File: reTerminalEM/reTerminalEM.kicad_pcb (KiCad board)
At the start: 2 copper layers, 135 x 90 mm, 7 parts, among them J1 FX23-100S-0.5SV

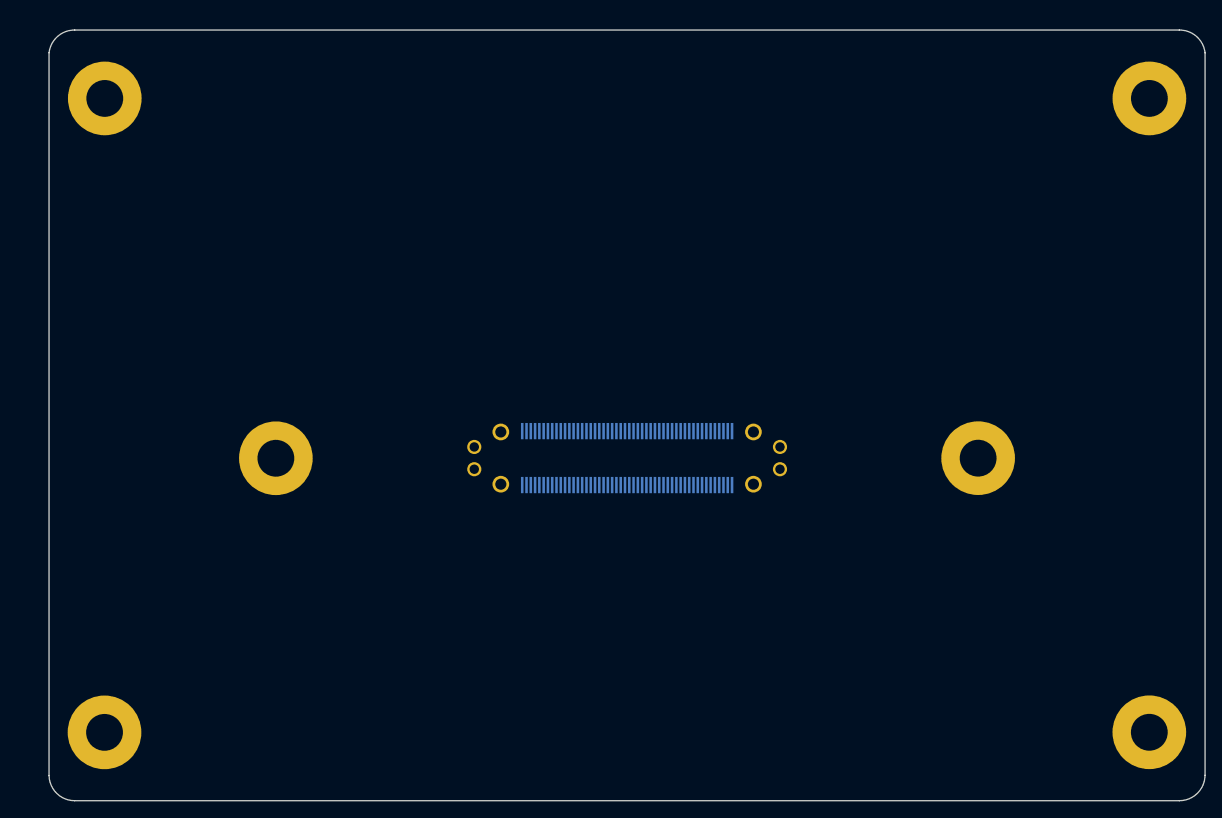
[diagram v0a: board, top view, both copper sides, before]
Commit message: fixing dimensions, adding .step, .dxf, .pdf
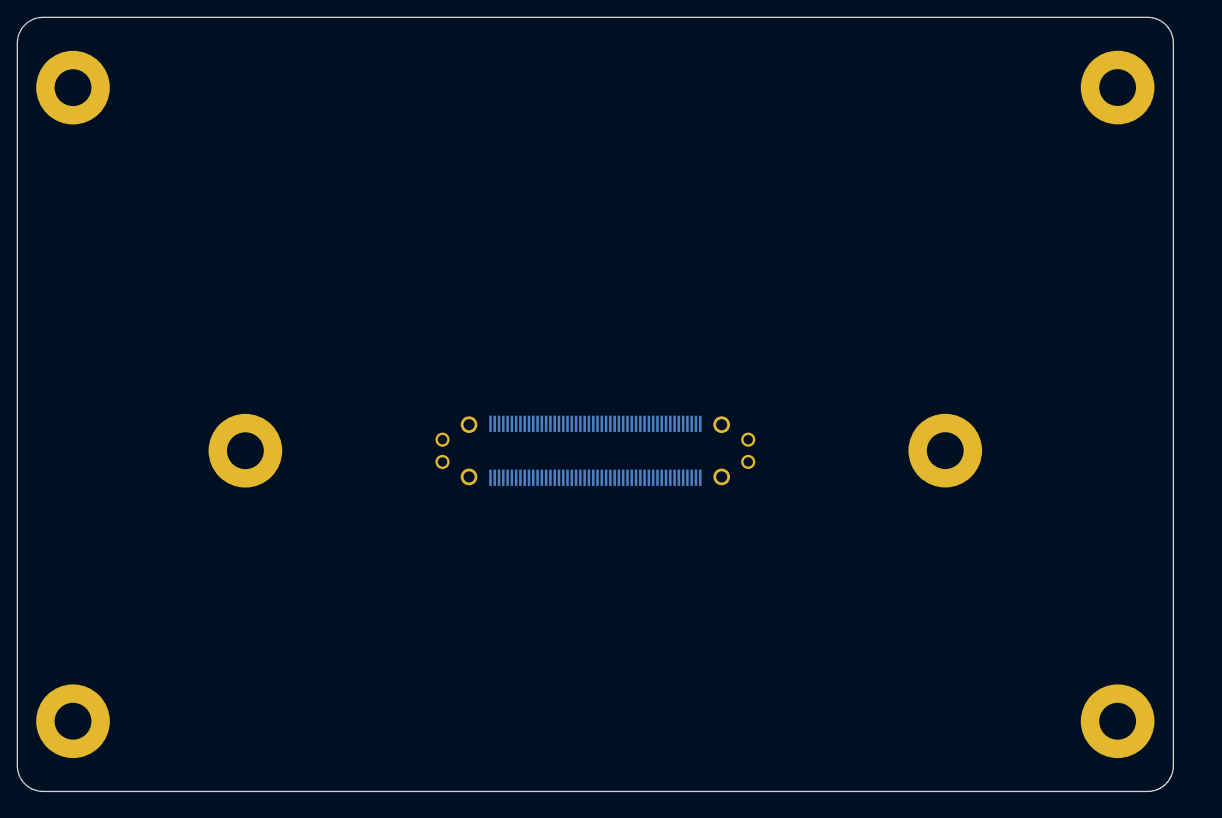
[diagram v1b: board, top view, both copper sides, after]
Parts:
- removed the REF** at (214.3, 136.8)
- removed the REF** at (214.3, 62.8)
- added REF**: MountingHole_4.3mm_M4_Pad, MountingHole:MountingHole_4.3mm_M4_Pad, F.Cu at (210.6, 135.5)
- added REF**: MountingHole_4.3mm_M4_Pad, MountingHole:MountingHole_4.3mm_M4_Pad, F.Cu at (210.6, 61.5)
- moved REF** 3.94 mm to (190.5, 103.9)
- moved REF** 3.92 mm to (88.6, 61.5)
- moved REF* 3.90 mm to (88.6, 135.5)
- moved J1 3.81 mm to (149.7, 103.9)
- moved REF** 3.67 mm to (108.7, 103.9)
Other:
- board size 135 x 90 mm -> 135 x 90.4 mm
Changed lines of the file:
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@@
   )
   (page A4)
+  (title_block
+    (date 2021-11-24)
+    (rev 0.1)
+    (company StanleyProjects.com)
+  )
   (layers
     (0 F.Cu signal)
@@
     (44 Edge.Cuts user)
     (45 Margin user)
-    (46 B.CrtYd user hide)
-    (47 F.CrtYd user hide)
+    (46 B.CrtYd user)
+    (47 F.CrtYd user)
     (48 B.Fab user hide)
     (49 F.Fab user hide)
@@
   )
   (module reTerminalModule:FX23-100S-0.5SV (layer B.Cu)
-    (at 153.37 104.77 180)
+    (at 149.6604 103.9196 180)
     (descr FX23-100S-0.5SV10-1)
     (tags Connector)
@@
   )
   (module MountingHole:MountingHole_4.3mm_M4_Pad locked (layer F.Cu)
-    (at 92.29 136.8)
+    (at 88.61 135.5)
     (descr "Mounting Hole 4.3mm, M4")
     (tags "mounting hole 4.3mm m4")
@@
   )
   (module MountingHole:MountingHole_4.3mm_M4_Pad locked (layer F.Cu)
-    (at 214.3 136.79)
+    (at 210.6 135.5)
     (descr "Mounting Hole 4.3mm, M4")
     (tags "mounting hole 4.3mm m4")
@@
   )
   (module MountingHole:MountingHole_4.3mm_M4_Pad locked (layer F.Cu)
-    (at 214.31 62.77)
+    (at 210.6 61.5)
     (descr "Mounting Hole 4.3mm, M4")
     (tags "mounting hole 4.3mm m4")
@@
   )
   (module MountingHole:MountingHole_4.3mm_M4_Pad locked (layer F.Cu)
-    (at 92.32 62.77)
+    (at 88.61 61.51)
     (descr "Mounting Hole 4.3mm, M4")
     (tags "mounting hole 4.3mm m4")
@@
   )
   (module MountingHole:MountingHole_4.3mm_M4_Pad locked (layer F.Cu)
-    (at 194.36 104.78)
+    (at 190.52 103.9)
     (descr "Mounting Hole 4.3mm, M4")
     (tags "mounting hole 4.3mm m4")
@@
   )
   (module MountingHole:MountingHole_4.3mm_M4_Pad locked (layer F.Cu)
-    (at 112.3 104.79)
+    (at 108.74 103.91)
     (descr "Mounting Hole 4.3mm, M4")
     (tags "mounting hole 4.3mm m4")
@@
     (pad 1 thru_hole circle (at 0.05 0) (size 8.6 8.6) (drill 4.3) (layers *.Cu *.Mask))
   )
-  (gr_circle (center 92.36 62.782045) (end 94.5 62.782045) (layer Eco1.User) (width 0.05))
-  (gr_circle (center 112.36 104.782045) (end 114.5 104.782045) (layer Eco1.User) (width 0.05))
-  (gr_circle (center 168.11 107.832045) (end 168.76 107.832045) (layer Eco1.User) (width 0.05))
-  (gr_circle (center 171.21 106.082045) (end 171.76 106.082045) (layer Eco1.User) (width 0.05))
-  (gr_circle (center 214.36 62.782045) (end 216.5 62.782045) (layer Eco1.User) (width 0.05))
-  (gr_circle (center 135.51 106.082045) (end 136.06 106.082045) (layer Eco1.User) (width 0.05))
-  (gr_line (start 88.86 144.782045) (end 217.8434 144.782045) (layer Edge.Cuts) (width 0.05))
-  (gr_arc (start 88.840171 57.781969) (end 88.86 54.782045) (angle -83.78911387) (layer Edge.Cuts) (width 0.05))
-  (gr_circle (center 92.36 136.782045) (end 94.5 136.782045) (layer Eco1.User) (width 0.05))
-  (gr_circle (center 171.21 103.482045) (end 171.76 103.482045) (layer Eco1.User) (width 0.05))
-  (gr_circle (center 138.61 107.832045) (end 139.26 107.832045) (layer Eco1.User) (width 0.05))
-  (gr_arc (start 217.879829 57.781972) (end 220.86 57.4377) (angle -83.78142973) (layer Edge.Cuts) (width 0.05))
-  (gr_line (start 85.86 57.4377) (end 85.86 141.838) (layer Edge.Cuts) (width 0.05))
-  (gr_arc (start 217.850431 141.772103) (end 217.8434 144.782044) (angle -89.22206063) (layer Edge.Cuts) (width 0.05))
-  (gr_line (start 217.8604 54.782045) (end 88.86 54.782045) (layer Edge.Cuts) (width 0.05))
-  (gr_circle (center 135.51 103.482045) (end 136.06 103.482045) (layer Eco1.User) (width 0.05))
-  (gr_circle (center 168.11 101.732045) (end 168.76 101.732045) (layer Eco1.User) (width 0.05))
-  (gr_circle (center 194.36 104.782045) (end 196.5 104.782045) (layer Eco1.User) (width 0.05))
-  (gr_arc (start 88.859468 141.782055) (end 85.86 141.838) (angle -88.94161501) (layer Edge.Cuts) (width 0.05))
-  (gr_circle (center 138.61 101.732045) (end 139.26 101.732045) (layer Eco1.User) (width 0.05))
-  (gr_circle (center 214.36 136.782045) (end 216.5 136.782045) (layer Eco1.User) (width 0.05))
-  (gr_line (start 220.86 141.82) (end 220.86 57.4377) (layer Edge.Cuts) (width 0.05))
+  (gr_circle (center 167.5052 102.636645) (end 168.0552 102.636645) (layer Eco1.User) (width 0.05))
+  (gr_circle (center 167.5052 105.236645) (end 168.0552 105.236645) (layer Eco1.User) (width 0.05))
+  (gr_circle (center 88.658973 61.5) (end 90.758973 61.5) (layer Eco1.User) (width 0.05))
+  (gr_line (start 85.158973 143.7) (end 214.158973 143.7) (layer Edge.Cuts) (width 0.05))
+  (gr_arc (start 85.158973 140.7) (end 82.158973 140.7) (angle -90) (layer Edge.Cuts) (width 0.05))
+  (gr_circle (center 88.658973 135.5) (end 90.758973 135.5) (layer Eco1.User) (width 0.05))
+  (gr_line (start 217.158973 140.7) (end 217.158973 56.3) (layer Edge.Cuts) (width 0.05))
+  (gr_arc (start 214.158973 56.3) (end 217.158973 56.3) (angle -90) (layer Edge.Cuts) (width 0.05))
+  (gr_line (start 82.158973 56.3) (end 82.158973 140.7) (layer Edge.Cuts) (width 0.05))
+  (gr_circle (center 210.658973 135.5) (end 212.758973 135.5) (layer Eco1.User) (width 0.05))
+  (gr_line (start 214.158973 53.3) (end 85.158973 53.3) (layer Edge.Cuts) (width 0.05))
+  (gr_arc (start 85.158973 56.3) (end 85.158973 53.3) (angle -90) (layer Edge.Cuts) (width 0.05))
+  (gr_circle (center 190.522946 103.9) (end 192.622946 103.9) (layer Eco1.User) (width 0.05))
+  (gr_arc (start 214.158973 140.7) (end 214.158973 143.7) (angle -90) (layer Edge.Cuts) (width 0.05))
+  (gr_circle (center 210.658973 61.5) (end 212.758973 61.5) (layer Eco1.User) (width 0.05))
+  (gr_circle (center 108.795 103.9) (end 110.895 103.9) (layer Eco1.User) (width 0.05))
+  (gr_circle (center 164.4052 106.976645) (end 165.0552 106.976645) (layer Eco1.User) (width 0.05))
+  (gr_circle (center 131.8052 105.226645) (end 132.3552 105.226645) (layer Eco1.User) (width 0.05))
+  (gr_circle (center 134.9052 106.976645) (end 135.5552 106.976645) (layer Eco1.User) (width 0.05))
+  (gr_circle (center 131.8052 102.626645) (end 132.3552 102.626645) (layer Eco1.User) (width 0.05))
+  (gr_circle (center 164.4052 100.876645) (end 165.0552 100.876645) (layer Eco1.User) (width 0.05))
+  (gr_circle (center 134.9052 100.876645) (end 135.5552 100.876645) (layer Eco1.User) (width 0.05))
 )
